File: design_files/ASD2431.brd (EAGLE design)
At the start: 28.3 x 26.3 mm, 39 parts, among them J1 EVP-ANDA1A, J2 DF12-32-DS, J3 EVP-ANDA1A, J4 EVP-ANDA1A, J5 EVP-ANDA1A, U1 XC6217A33, U2 TXB0104, U3 UG-9664HDDAG01, U4 FAN5331SX, U5 SX1505I087TRT

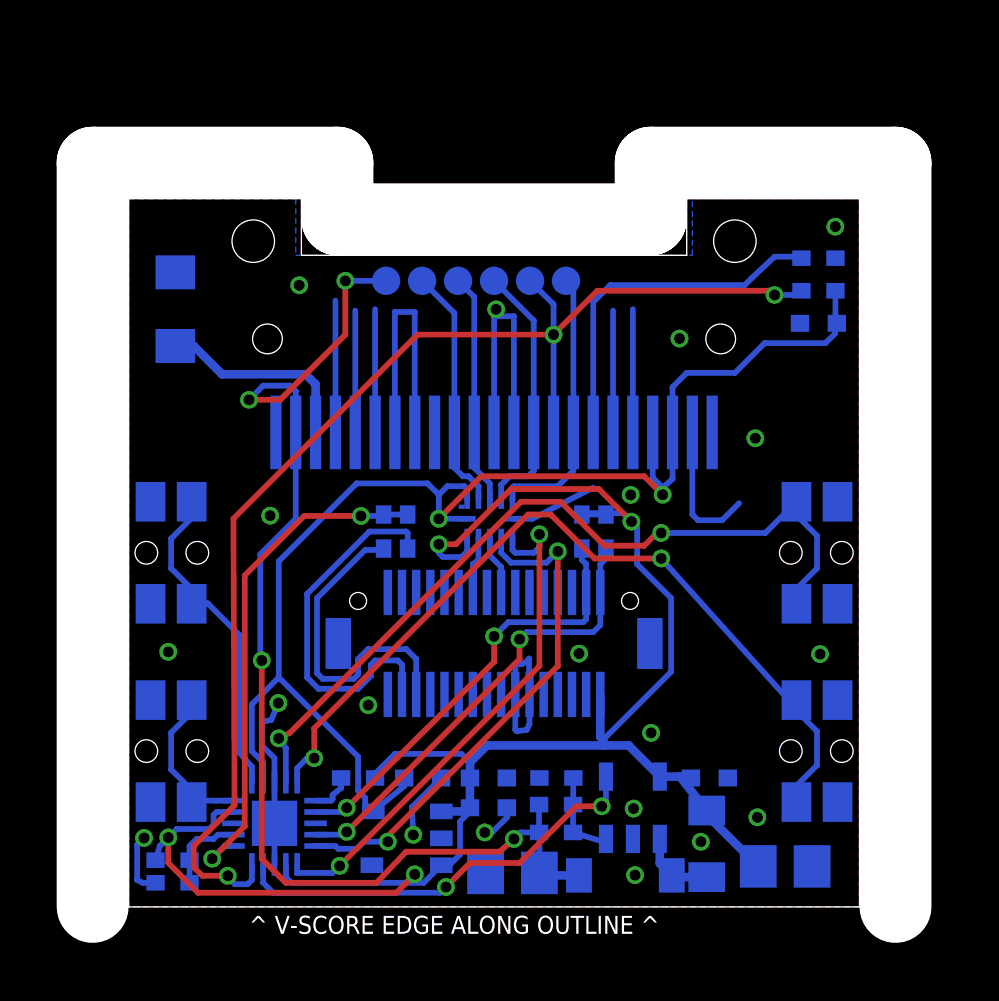
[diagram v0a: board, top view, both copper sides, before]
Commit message: update files
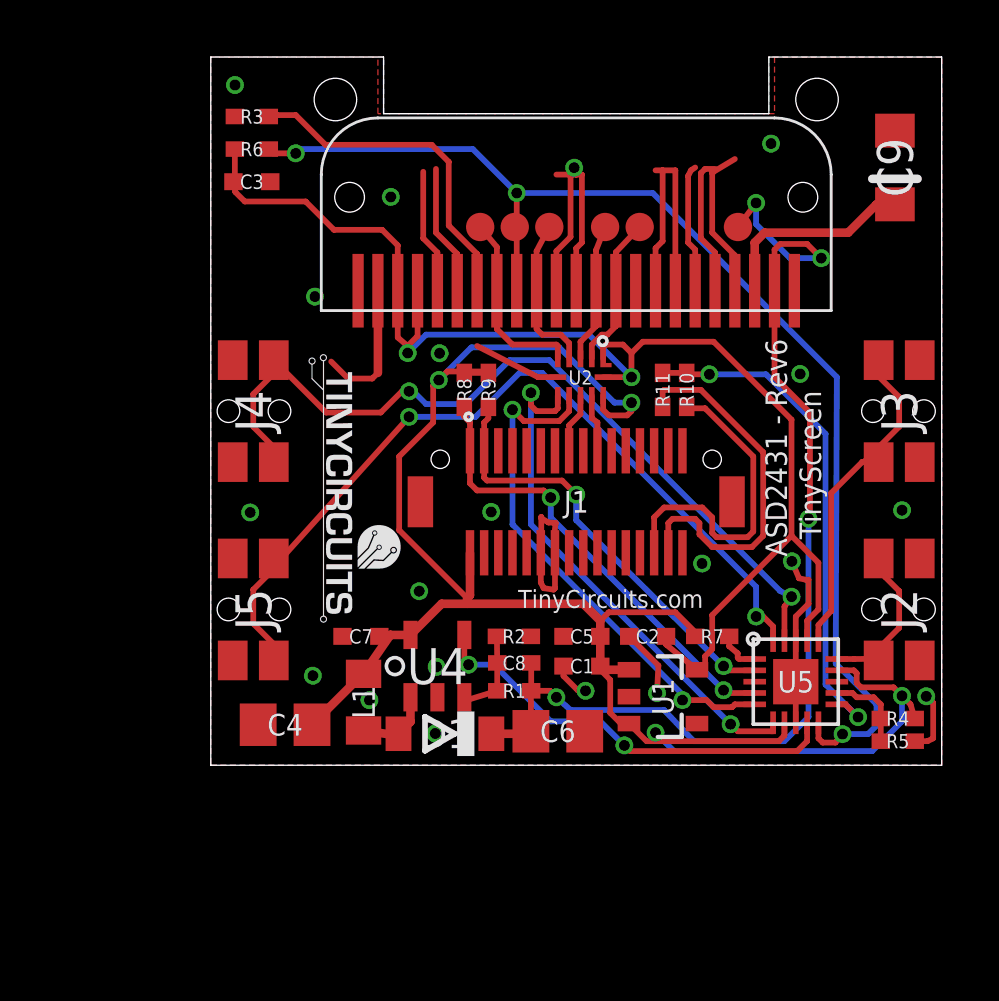
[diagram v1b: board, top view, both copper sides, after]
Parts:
- removed C15: 4.7uF, tinycircuits:1206_CAP_TANT
- added C8: 100pF, tinycircuits:0402
- C9: value 180pF -> 4.7uF; device tinycircuits:0402 -> tinycircuits:1206_CAP_TANT
- J1: value EVP-ANDA1A -> DF12-32-DS; device tinycircuits:PTS840GKP -> tinycircuits:DF12-32-DS
- J2: value DF12-32-DS -> EVP-ANDA1A; device tinycircuits:DF12-32-DS -> tinycircuits:PTS840GKP
- R1: value 100K -> 200K
- R2: value 10.0K -> 22.0K
- R3: value 1.00M -> 1.2M
- moved J3 26.2 mm to (34.3, 22.5), flipped to the top
- moved R4 26.1 mm to (34.2, 11.7), flipped to the top
- moved R5 26.1 mm to (34.2, 10.8), flipped to the top
- moved C9 25.5 mm to (34.1, 31.1), flipped to the top, turned to 90 degrees
- moved J4 23.2 mm to (11.5, 22.5), flipped to the top
- moved C3 20.6 mm to (11.4, 30.6), flipped to the top
- moved R3 20.6 mm to (11.4, 32.9), flipped to the top
- moved R6 20.6 mm to (11.4, 31.8), flipped to the top
- moved J5 20.0 mm to (11.5, 15.5), flipped to the top
- moved U5 19.1 mm to (30.6, 12.9), flipped to the top
- moved C4 18.3 mm to (12.6, 11.4), flipped to the top
- moved J1 16.8 mm to (22.9, 19.3), flipped to the top, turned to 0 degrees
- moved J2 14.4 mm to (34.3, 15.5), flipped to the top, turned to 90 degrees
- moved R7 13.5 mm to (27.7, 14.6), flipped to the top
- moved C7 13.3 mm to (15.3, 14.6), flipped to the top
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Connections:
- net +12V: now also C8.1; no longer C9.1
- net +3V3: now also J1.6; no longer J2.6
- net +5V: now also J1.8; no longer J2.8
- net AD0: now also J1.11; no longer J2.11
- net AD1: now also J1.9; no longer J2.9
- net AD2: now also J1.7; no longer J2.7
- net AD3: now also J1.5; no longer J2.5
- net AD4/SDA: now also J1.3; no longer J2.3
- net AD5/SCL: now also J1.1; no longer J2.1
- net AREF: now also J1.13; no longer J2.13
- net BTN0: now also J2.1, J2.2; no longer J1.1, J1.2
- net BTN2: now also J4.1, J4.2; no longer J5.1, J5.2
- net BTN3: now also J5.1, J5.2; no longer J4.1, J4.2
- net GND: now also C9.2, J1.12, J1.14, J2.3, J2.4; no longer C15.2, J1.3, J1.4, J2.12, J2.14
- net IO0: now also J1.24; no longer J2.24
- net IO1: now also J1.26; no longer J2.26
- net IO2: now also J1.28; no longer J2.28
- net IO3: now also J1.30; no longer J2.30
- net IO4: now also J1.32; no longer J2.32
- net IO5: now also J1.31; no longer J2.31
- net IO6: now also J1.29; no longer J2.29
- net IO7: now also J1.27; no longer J2.27
- net IO8: now also J1.25; no longer J2.25
- net IO9: now also J1.23; no longer J2.23
- net MISO: now also J1.17; no longer J2.17
- net MOSI: now also J1.19; no longer J2.19
- net N$3: now also C8.2; no longer C9.2
- net N$7: now also C9.1; no longer C15.1
- net RESET: now also J1.22; no longer J2.22
- net RSV0: now also J1.20; no longer J2.20
- net RSV1: now also J1.18; no longer J2.18
- net RSV2: now also J1.16; no longer J2.16
- net SCK: now also J1.15; no longer J2.15
- net SS: now also J1.21; no longer J2.21
- net VBATT: now also J1.4; no longer J2.4
- net VCC: now also J1.2; no longer J2.2
- net VIN: now also J1.10; no longer J2.10
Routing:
- net D/C#: track 9.19 -> 5.62 mm
- net SCLK: track 8.21 -> 4.94 mm
- net SDIN: track 8.69 -> 5.45 mm
- net +12V: track 41.4 -> 38.4 mm
- net CS#: track 9.64 -> 6.66 mm
- net GND: track 65.9 -> 68.4 mm
- net RES#: track 45.0 -> 42.9 mm
- net BTN2: track 28.8 -> 29.4 mm
- net N$6: track 12.6 -> 12.0 mm
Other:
- board size 28.3 x 26.3 mm -> 25.8 x 25 mm
- board text added: "6"
- board text added: "ASD2431 - Rev6"
- board text added: "TinyCircuits.com"
- board text removed: "5"
- board text removed: "ASD2431 - Rev5"
- board text removed: "Tiny-Circuits.com"
- board text removed: "^ V-SCORE EDGE ALONG OUTLINE ^"
